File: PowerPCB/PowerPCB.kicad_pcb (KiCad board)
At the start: 4 copper layers, 100 x 60 mm, 81 parts, among them J1 Battery, J10 Conn_01x02, J2 Conn_01x02, J3 12Vout, J4 Conn_01x03, J5 5Vout, J6 Conn_01x03, J7 Conn_01x03, J8 Conn_01x02, J9 Conn_01x03, U1 TPS551892QWRYQRQ1, U2 FS1403-5000-AL

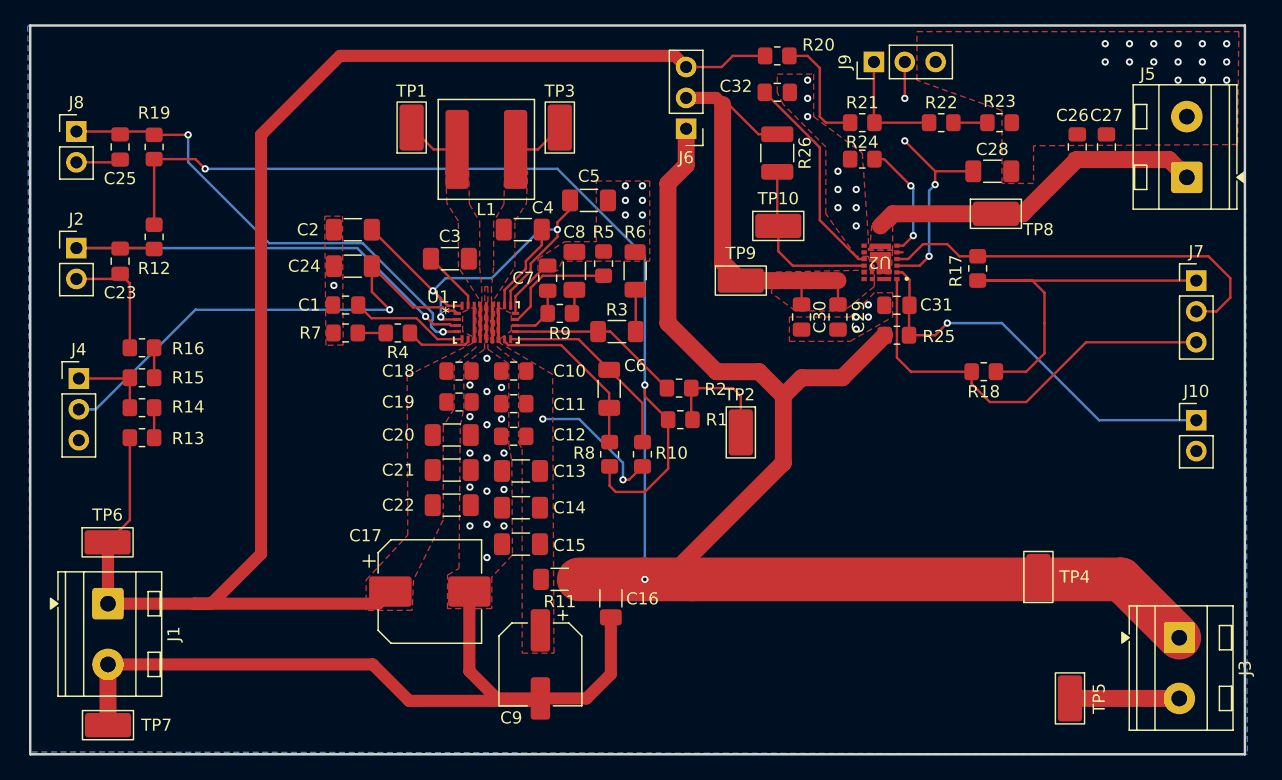
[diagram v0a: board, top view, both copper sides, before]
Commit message: PowerPCB v2
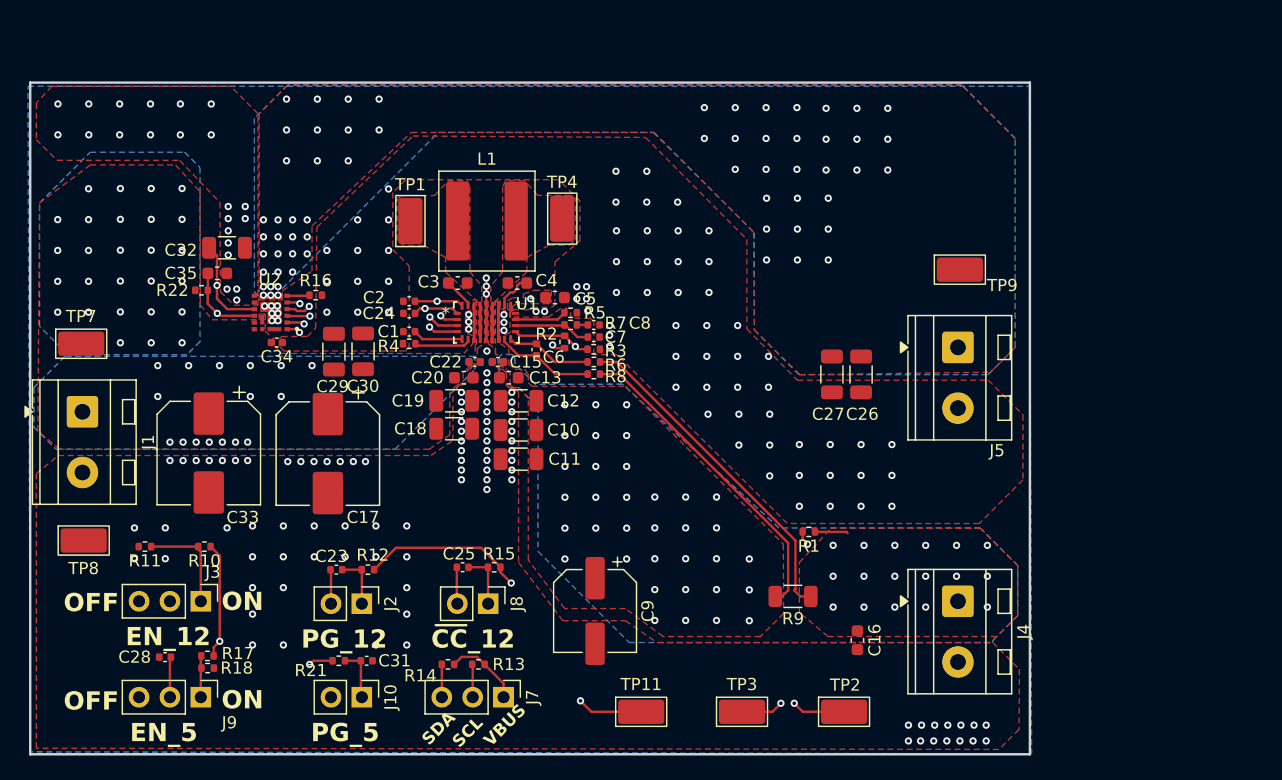
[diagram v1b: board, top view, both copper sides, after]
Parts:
- removed J6: Conn_01x03, Connector_PinHeader_2.54mm:PinHeader_1x03_P2.54mm_Vertical
- removed the R10 at (158.4, 101.3)
- removed the R14 at (117.2, 97.5)
- removed R19, R20, R23: 100k, Resistor_SMD:R_0805_2012Metric_Pad1.20x1.40mm_HandSolder
- removed R24: 0, Resistor_SMD:R_0805_2012Metric_Pad1.20x1.40mm_HandSolder
- removed the R6 at (157.8, 86.2)
- removed the R7 at (134.0, 91.3)
- removed the TP4 at (191.0, 111.4)
- removed TP5: TestPoint, TestPoint:TestPoint_Keystone_5019_Miniature
- removed the TP9 at (166.5, 87.0)
- added C33: 68uF, Capacitor_SMD:CP_Elec_8x10, F.Cu at (122.7, 101.2)
- added C34: 0.1uF, Capacitor_SMD:C_0402_1005Metric, F.Cu at (128.3, 92.1)
- added C35: 1uF, Capacitor_SMD:C_0603_1608Metric, F.Cu at (123.4, 86.4)
- added R16: 0, Resistor_SMD:R_0402_1005Metric, F.Cu at (131.5, 88.2)
- added R8: 10, Resistor_SMD:R_0402_1005Metric, F.Cu at (154.4, 94.7)
- added TP3: TestPoint, TestPoint:TestPoint_Keystone_5019_Miniature, F.Cu at (166.6, 122.5)
- C1, C23, C25, C31, C7: footprint Capacitor_SMD:C_0805_2012Metric_Pad1.18x1.45mm_HandSolder -> Capacitor_SMD:C_0402_1005Metric
- C10, C11, C12, C18, C19, C26, C27, C29, C30, C32: footprint Capacitor_SMD:C_0805_2012Metric_Pad1.18x1.45mm_HandSolder -> Capacitor_SMD:C_1206_3216Metric
- C13, C16, C20, C3, C4, C5: footprint Capacitor_SMD:C_1206_3216Metric_Pad1.33x1.80mm_HandSolder -> Capacitor_SMD:C_0603_1608Metric
- C14, C21: footprint Capacitor_SMD:C_1206_3216Metric_Pad1.33x1.80mm_HandSolder -> Capacitor_SMD:C_0402_1005Metric; moved to B.Cu
- C15, C2, C22, C24, C28, C6, C8: footprint Capacitor_SMD:C_1206_3216Metric_Pad1.33x1.80mm_HandSolder -> Capacitor_SMD:C_0402_1005Metric
- C9: footprint Capacitor_SMD:CP_Elec_6.3x5.4 -> Capacitor_SMD:CP_Elec_6.3x5.8
- R1: value 51 -> 49.9; footprint Resistor_SMD:R_0805_2012Metric_Pad1.20x1.40mm_HandSolder -> Resistor_SMD:R_0402_1005Metric
- R10: renamed from R13; value 100k -> 147k; footprint Resistor_SMD:R_0805_2012Metric_Pad1.20x1.40mm_HandSolder -> Resistor_SMD:R_0402_1005Metric
- R11: renamed from R16; value 100k -> 115k; footprint Resistor_SMD:R_0805_2012Metric_Pad1.20x1.40mm_HandSolder -> Resistor_SMD:R_0402_1005Metric
- R12, R2: value 100k -> 102k; footprint Resistor_SMD:R_0805_2012Metric_Pad1.20x1.40mm_HandSolder -> Resistor_SMD:R_0402_1005Metric
- R13: renamed from R17; value 47k -> 4.99k; footprint Resistor_SMD:R_0805_2012Metric_Pad1.20x1.40mm_HandSolder -> Resistor_SMD:R_0402_1005Metric
- R14: renamed from R18; value 47k -> 4.99k; footprint Resistor_SMD:R_0805_2012Metric_Pad1.20x1.40mm_HandSolder -> Resistor_SMD:R_0402_1005Metric
- R15: value 15k -> 102k; footprint Resistor_SMD:R_0805_2012Metric_Pad1.20x1.40mm_HandSolder -> Resistor_SMD:R_0402_1005Metric
- R17: renamed from R21; value 47k -> 49.9k; footprint Resistor_SMD:R_0805_2012Metric_Pad1.20x1.40mm_HandSolder -> Resistor_SMD:R_0402_1005Metric
- R18: renamed from R22; value 15k -> 12.7k; footprint Resistor_SMD:R_0805_2012Metric_Pad1.20x1.40mm_HandSolder -> Resistor_SMD:R_0402_1005Metric
- R21: renamed from R25; value 100k -> 49.9k; footprint Resistor_SMD:R_0805_2012Metric_Pad1.20x1.40mm_HandSolder -> Resistor_SMD:R_0402_1005Metric
- R22: renamed from R26; footprint Resistor_SMD:R_1210_3225Metric_Pad1.30x2.65mm_HandSolder -> Resistor_SMD:R_0402_1005Metric
- R3: value 5.6k -> 11.3k; footprint Resistor_SMD:R_1206_3216Metric_Pad1.30x1.75mm_HandSolder -> Resistor_SMD:R_0402_1005Metric
- R4: value 47k -> 49.9k; footprint Resistor_SMD:R_0805_2012Metric_Pad1.20x1.40mm_HandSolder -> Resistor_SMD:R_0402_1005Metric
- R5: value 120k -> 150k; footprint Resistor_SMD:R_0805_2012Metric_Pad1.20x1.40mm_HandSolder -> Resistor_SMD:R_0402_1005Metric
- R6: renamed from R8; footprint Resistor_SMD:R_0805_2012Metric_Pad1.20x1.40mm_HandSolder -> Resistor_SMD:R_0402_1005Metric
- R7: renamed from R9; footprint Resistor_SMD:R_0805_2012Metric_Pad1.20x1.40mm_HandSolder -> Resistor_SMD:R_0402_1005Metric
- R9: renamed from R11; footprint Resistor_SMD:R_1206_3216Metric_Pad1.30x1.75mm_HandSolder -> Resistor_SMD:R_1206_3216Metric
- moved C28 79.0 mm to (119.1, 118.0)
- moved J9 76.2 mm to (122.0, 121.3), turned to -90 degrees
- moved R18 75.3 mm to (122.6, 118.9)
- moved J10 72.4 mm to (135.3, 121.3), turned to -90 degrees
- moved R17 69.5 mm to (122.6, 117.9), turned to 180 degrees
- moved J7 66.6 mm to (147.0, 121.3), turned to -90 degrees
- moved R21 53.2 mm to (133.4, 118.3)
- moved C31 52.6 mm to (135.7, 118.3), turned to 0 degrees
- moved R13 52.5 mm to (144.9, 118.6), turned to 180 degrees
- moved J8 51.6 mm to (145.7, 113.6), turned to -90 degrees
- moved U2 50.4 mm to (127.8, 89.6)
- moved R14 50.3 mm to (142.4, 118.6)
- moved R22 48.7 mm to (122.1, 87.8), turned to 0 degrees
- moved C32 47.1 mm to (124.2, 84.3)
- moved C25 44.6 mm to (143.6, 110.6), turned to 0 degrees
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- renumbered J4 to J3, J3 to J4, TP10 to TP11, TP3 to TP4, TP6 to TP7, TP7 to TP8, TP8 to TP9
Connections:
- net Net-(U1A-DITH/SYNC) renamed /DITH/SYNC
- C1 pad 1: V_BAT- -> GND
- C10 pad 1: Net-(U1A-VOUT) -> V_OUT_12+
- C10 pad 2: V_BAT- -> GND
- C11 pad 1: Net-(U1A-VOUT) -> V_OUT_12+
- C11 pad 2: V_BAT- -> GND
- C12 pad 1: Net-(U1A-VOUT) -> V_OUT_12+
- C12 pad 2: V_BAT- -> GND
- C13 pad 1: Net-(U1A-VOUT) -> V_OUT_12+
- C13 pad 2: V_BAT- -> GND
- C14 pad 1: Net-(U1A-VOUT) -> V_OUT_12+
- C14 pad 2: V_BAT- -> GND
- C15 pad 1: Net-(U1A-VOUT) -> V_OUT_12+
- C15 pad 2: V_BAT- -> GND
- C16 pad 2: V_BAT- -> GND
- C17 pad 2: V_BAT- -> GND
- C18 pad 2: V_BAT- -> GND
- C19 pad 2: V_BAT- -> GND
- C2 pad 1: V_BAT- -> GND
- C20 pad 2: V_BAT- -> GND
- C21 pad 2: V_BAT- -> GND
- C22 pad 2: V_BAT- -> GND
- C23 pad 1: PG_12 -> GND
- C23 pad 2: V_BAT- -> PG_12
- C24 pad 1: EN_12 -> GND
- C24 pad 2: V_BAT- -> EN_12
- C25 pad 1: *CC_12 -> GND
- C25 pad 2: V_BAT- -> *CC_12
- C26 pad 2: V_BAT- -> GND
- C27 pad 2: V_BAT- -> GND
- C28 pad 1: EN_5 -> GND
- C28 pad 2: V_BAT- -> EN_5
- C29 pad 1: 12V_IN -> V_BAT+
- C29 pad 2: V_BAT- -> GND
- C30 pad 1: 12V_IN -> V_BAT+
- C30 pad 2: V_BAT- -> GND
- C31 pad 2: V_BAT- -> GND
- C32 pad 1: Net-(U2-VCC) -> /VCC_5
- C32 pad 2: V_BAT- -> GND
- C5 pad 2: V_BAT- -> GND
- C7 pad 2: V_BAT- -> GND
- C8 pad 2: V_BAT- -> GND
- C9 pad 1: Net-(U1A-VOUT) -> V_OUT_12+
- C9 pad 2: V_BAT- -> GND
- J1 pad 2: V_BAT- -> GND
- J10 pad 2: V_BAT- -> GND
- J2 pad 2: V_BAT- -> GND
- J3 pad 1: Net-(J4-Pin_1) -> Net-(J3-Pin_1)
- J3 pad 3: V_BAT- -> GND
- J4 pad 2: V_BAT- -> GND
- J5 pad 2: V_BAT- -> GND
- J8 pad 2: V_BAT- -> GND
- J9 pad 3: V_BAT- -> GND
- R10 pad 2: Net-(R13-Pad2) -> Net-(J3-Pin_1)
- R11 pad 1: Net-(R15-Pad2) -> Net-(J3-Pin_1)
- R11 pad 2: V_BAT- -> GND
- R12 pad 1: V_OUT_12+ -> PG_12
- R12 pad 2: PG_12 -> VCC_12
- R15 pad 1: Net-(J4-Pin_1) -> *CC_12
- R15 pad 2: Net-(R15-Pad2) -> VCC_12
- R17 pad 1: Net-(R20-Pad2) -> V_BAT+
- R18 pad 2: Net-(R22-Pad2) -> GND
- R21 pad 1: V_OUT_12+ -> /VCC_5
- R22 pad 1: 12V_IN -> V_BAT+
- R3 pad 1: Net-(R3-Pad1) -> GND
- R4 pad 2: Net-(R4-Pad2) -> GND
- R5 pad 2: V_BAT- -> GND
- R6 pad 2: Net-(U1A-ISP) -> Net-(U1A-ISN)
- R9 pad 2: Net-(U1A-VOUT) -> V_OUT_12+
- TP8 pad 1: V_BAT- -> GND
- U1 pad 11: Net-(U1A-VOUT) -> V_OUT_12+
- U1 pad 17: V_BAT- -> GND
- U1 pad 9: V_BAT- -> GND
- U2 pad 10: Net-(U2-VCC) -> /VCC_5
- U2 pad 12: 12V_IN -> V_BAT+
- U2 pad 13: 12V_IN -> V_BAT+
- U2 pad 14: 12V_IN -> V_BAT+
- U2 pad 16: V_BAT- -> GND
- U2 pad 17: 12V_IN -> V_BAT+
- U2 pad 8: V_BAT- -> GND
- U2 pad 9: V_BAT- -> GND
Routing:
- net V_OUT_12+: track 202.2 -> 57.0 mm, vias 3 -> 55
- net V_BAT-: track 121.5 -> 0.00 mm, vias 52 -> 0
- net V_BAT+: track 124.7 -> 45.2 mm, vias 0 -> 47
- net /VCC_5: track 0.00 -> 71.7 mm, vias 0 -> 2
- net Net-(U2-VIN): track 14.0 -> 71.1 mm, vias 0 -> 2
- net Net-(R1-Pad2): track 9.85 -> 51.1 mm, vias 0 -> 3
- net Net-(U1A-FB): track 14.4 -> 50.9 mm, vias 0 -> 2
- net 12V_IN: track 35.8 -> 0.00 mm
- net VBUS: track 33.5 -> 6.36 mm
- net V_OUT_5+: track 28.6 -> 3.18 mm, vias 0 -> 62
- net EN_5: track 23.4 -> 47.9 mm, vias 4 -> 1
- net PG_5: track 33.2 -> 57.0 mm
- net Net-(U2-VCC): track 17.4 -> 0.00 mm
- net VCC_12: track 36.1 -> 52.6 mm, vias 3 -> 4
- net Net-(U1A-VOUT): track 11.5 -> 0.00 mm, vias 2 -> 0
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- added copper zone on B.Cu, net GND
- added copper zone on F.Cu, net GND
- added copper zone on In2.Cu, net GND
- added copper zone on F.Cu, net VCC_12
- added copper zone on B.Cu, net V_BAT+
- added copper zone on B.Cu, net V_OUT_12+
- added copper zone on F.Cu, net V_OUT_12+
- added copper zone on B.Cu, net V_OUT_5+
- removed copper zone on F.Cu, net 12V_IN
- removed copper zone on F.Cu, net Net-(U1A-VOUT)
- removed copper zone on B.Cu, net V_BAT-
- removed copper zone on F.Cu, net V_BAT-
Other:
- board size 100 x 60 mm -> 82.3 x 55.3 mm
- board text added: "CC_12"
- board text added: "EN_12"
- board text added: "EN_5"
- board text added: "OFF"
- board text added: "ON"
- board text added: "PG_12"
- board text added: "PG_5"
- board text added: "SCL"
- board text added: "SDA"
- board text added: "VBUS"
- board text removed: "${REFERENCE}"
